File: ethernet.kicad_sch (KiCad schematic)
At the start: 57 parts, among them J9 Bus_RJ45_7499111121A, U9 KSZ9031RNXCA, Y1 Oscillator_SMD_25MHz_KX-7

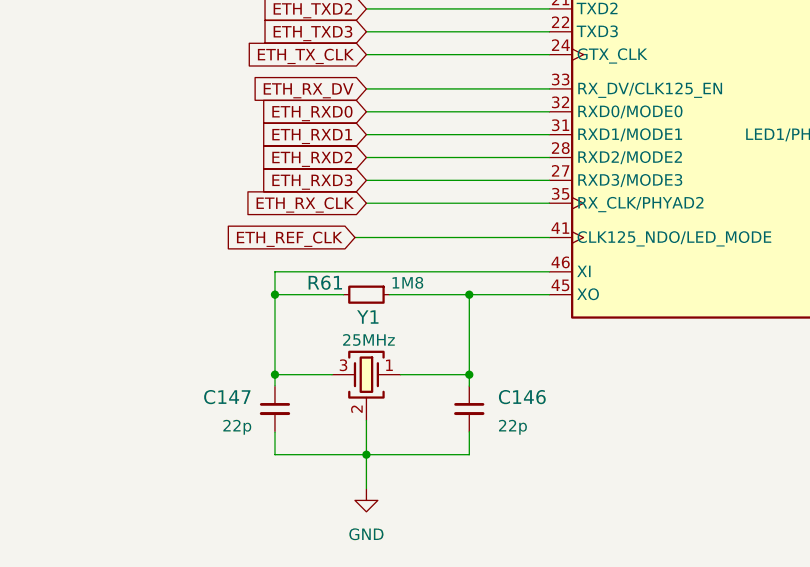
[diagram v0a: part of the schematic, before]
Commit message: [#87036] Update R61
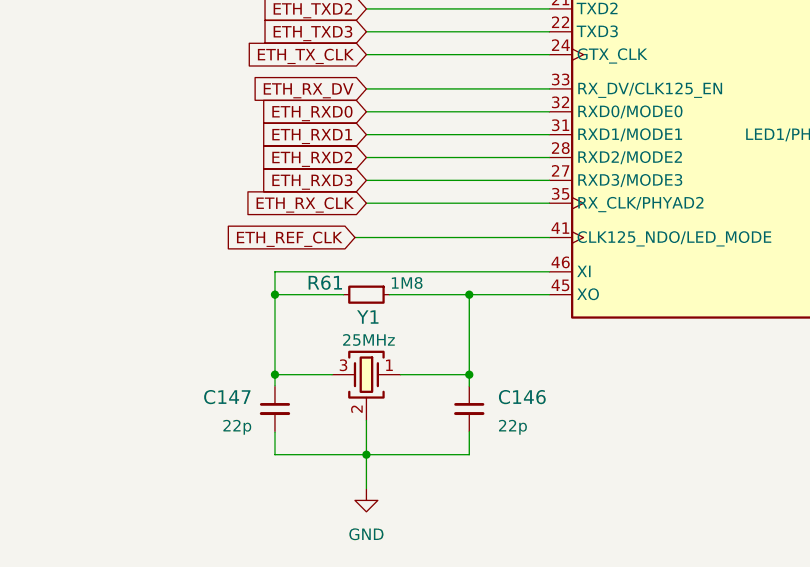
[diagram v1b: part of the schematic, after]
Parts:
- R61: symbol antmicroResistors0402:R_1M8_5%_0402 -> antmicroResistors0402:R_1M8_0402; MPN MCMR04X185_JTL -> RC0402FR-071M8L; Manufacturer Multicomp Pro -> YAGEO; Tolerance 5% -> 1%
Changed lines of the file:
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@@
 	)
 	(symbol
-		(lib_id "antmicroResistors0402:R_1M8_5%_0402")
+		(lib_id "antmicroResistors0402:R_1M8_0402")
 		(at 194.31 116.84 0)
 		(mirror y)
@@
 			)
 		)
-		(property "Datasheet" "https://www.farnell.com/datasheets/2860635.pdf"
+		(property "Datasheet" "https://www.mouser.com/catalog/specsheets/YAGEO_PYu_RC_Group_51_RoHS_L_12.pdf"
 			(at 173.99 134.62 0)
 			(effects
@@
 			)
 		)
-		(property "Description" "SMD Chip Resistor, Ceramic, 1.8 Mohm, ± 5%, 62.5 mW, 0402 [1005 Metric], Thick Film"
+		(property "Description" "SMD Chip Resistor"
 			(at 173.99 147.32 0)
 			(effects
@@
 			)
 		)
-		(property "Manufacturer" "Multicomp Pro"
+		(property "Manufacturer" "YAGEO"
 			(at 173.99 139.7 0)
 			(effects
@@
 			)
 		)
-		(property "MPN" "MCMR04X185_JTL"
+		(property "MPN" "RC0402FR-071M8L"
 			(at 173.99 137.16 0)
 			(effects
@@
 		)
 		(property "Val" "1M8"
-			(at 196.342 115.57 0)
+			(at 198.12 116.332 0)
 			(effects
 				(font
@@
 					(thickness 0.15)
 				)
+				(justify left bottom)
 			)
 		)
@@
 			)
 		)
-		(property "Tolerance" "5%"
+		(property "Tolerance" "1%"
 			(at 173.99 127 0)
 			(effects
